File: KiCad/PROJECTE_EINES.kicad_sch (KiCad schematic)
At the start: 7 parts

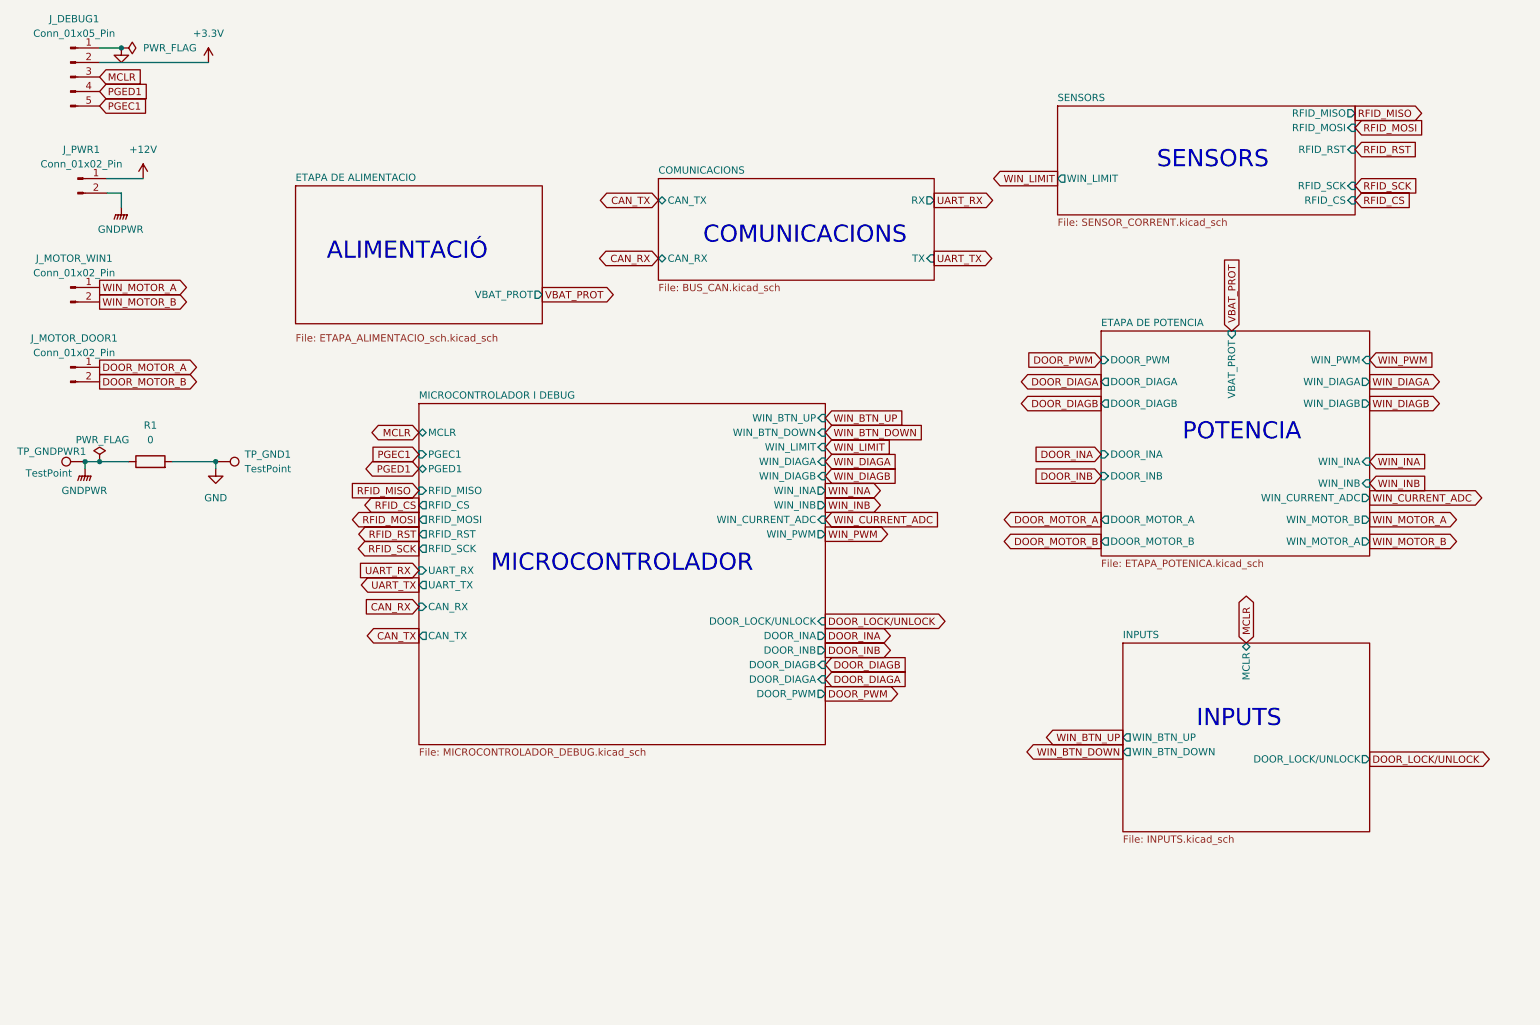
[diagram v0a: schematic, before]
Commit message: Versio final KiCad, BOM i Diagrama de Blocs
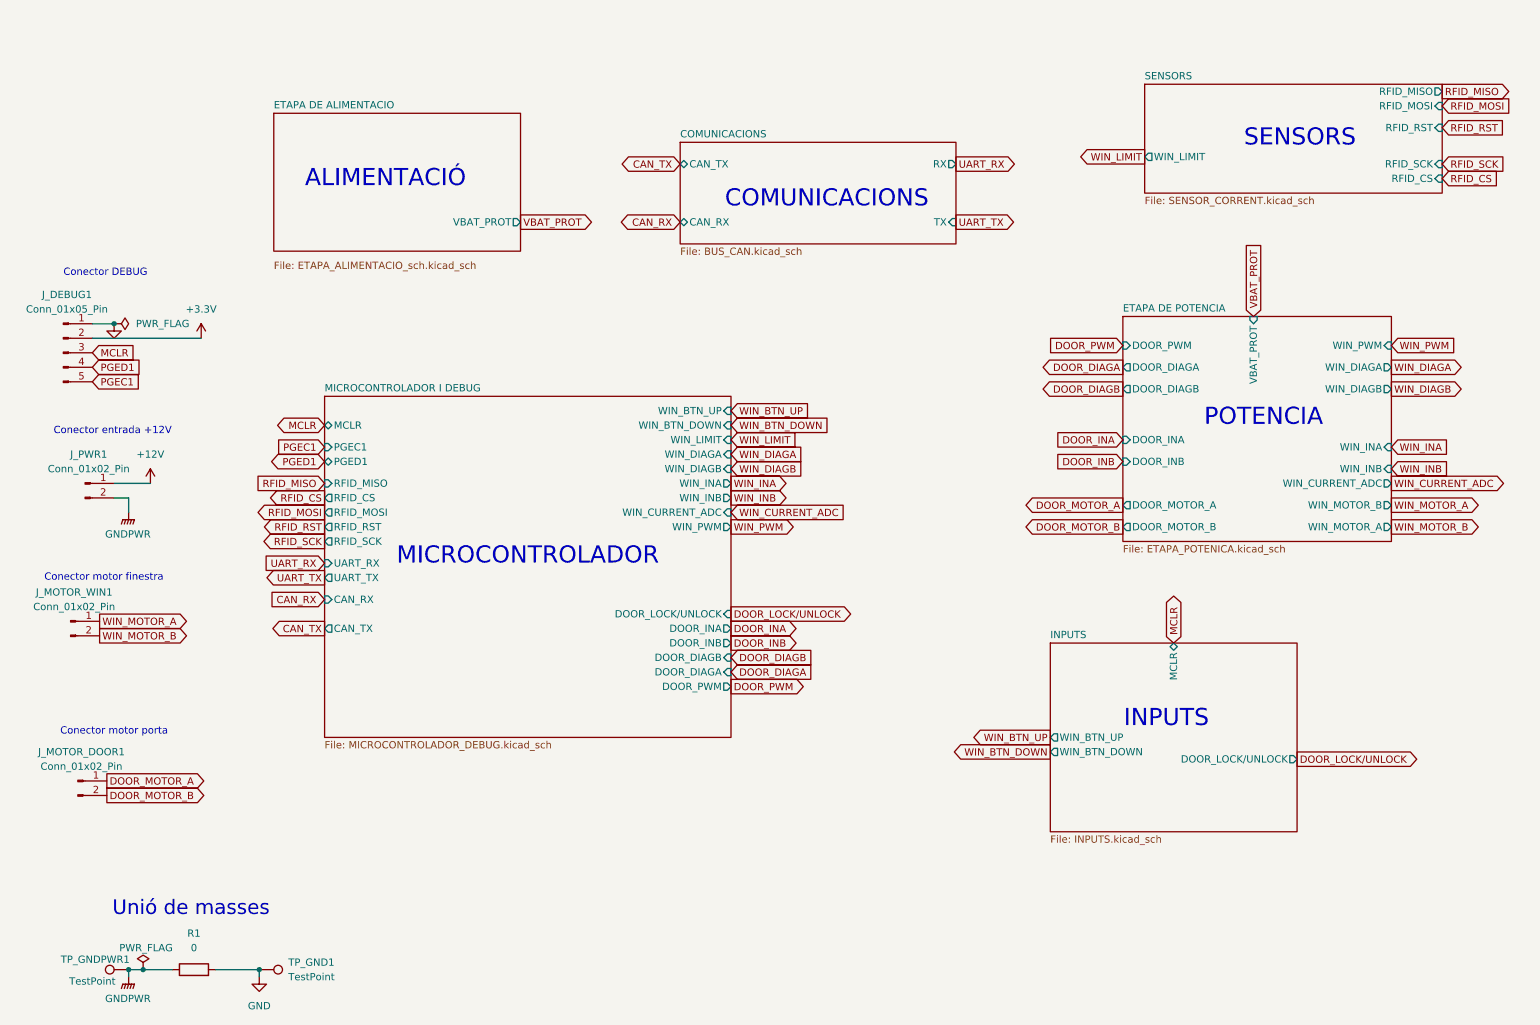
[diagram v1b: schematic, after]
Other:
- note added: "Conector DEBUG"
- note added: "Conector entrada +12V"
- note added: "Conector motor finestra"
- note added: "Conector motor porta"
- note added: "Unió de masses"
- moved on the sheet: J_DEBUG1, J_MOTOR_DOOR1, J_MOTOR_WIN1, J_PWR1, R1, TP_GND1, TP_GNDPWR1
